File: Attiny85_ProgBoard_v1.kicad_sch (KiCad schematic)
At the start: 1 part, among them U1 ATtiny85V-10PU

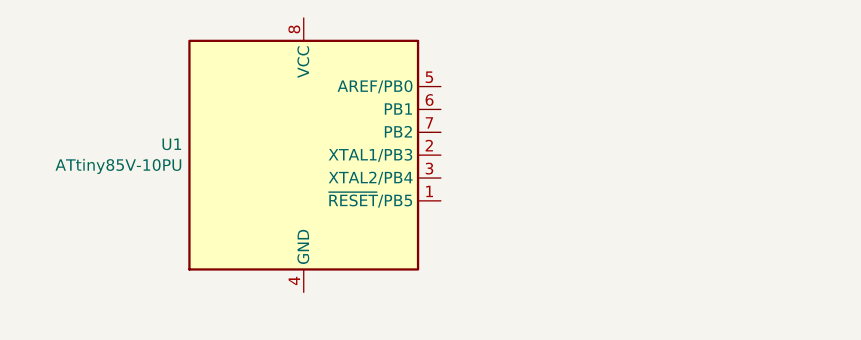
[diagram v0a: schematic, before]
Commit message: Designed PCB
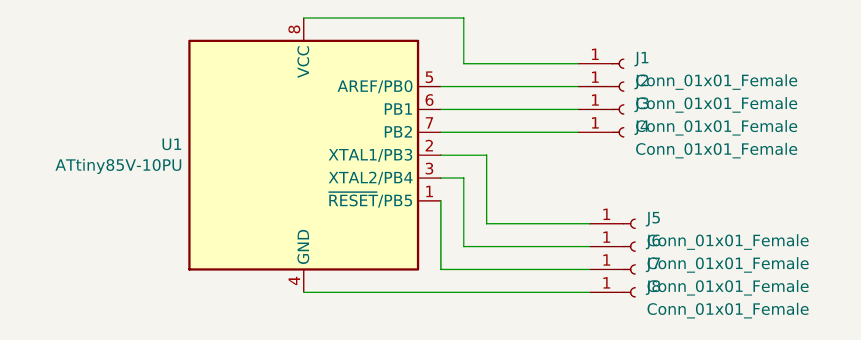
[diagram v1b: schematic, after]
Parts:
- added J1, J2, J3, J4, J5, J6, J7, J8: Conn_01x01_Female, Connector_Pin:PinHole_01x01, symbol Connector:Conn_01x01_Female
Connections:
- net at U1.1 (~{RESET}/PB5): now also J7.1 (Pin_1)
- net at U1.2 (XTAL1/PB3): now also J5.1 (Pin_1)
- net at U1.3 (XTAL2/PB4): now also J6.1 (Pin_1)
- net at U1.4 (GND): now also J8.1 (Pin_1)
- net at U1.5 (AREF/PB0): now also J2.1 (Pin_1)
- net at U1.6 (PB1): now also J3.1 (Pin_1)
- net at U1.7 (PB2): now also J4.1 (Pin_1)
- net at U1.8 (VCC): now also J1.1 (Pin_1)
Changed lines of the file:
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@@
 (kicad_sch (version 20230121) (generator eeschema)
   (paper "A4")
+  (wire (pts (xy 120.65 60.96) (xy 138.43 60.96))
+    (stroke (width 0) (type default))
+  )
+  (wire (pts (xy 135.89 71.12) (xy 151.13 71.12))
+    (stroke (width 0) (type default))
+  )
+  (wire (pts (xy 138.43 78.74) (xy 135.89 78.74))
+    (stroke (width 0) (type default))
+  )
+  (wire (pts (xy 135.89 88.9) (xy 152.4 88.9))
+    (stroke (width 0) (type default))
+  )
+  (wire (pts (xy 152.4 86.36) (xy 138.43 86.36))
+    (stroke (width 0) (type default))
+  )
+  (wire (pts (xy 135.89 76.2) (xy 140.97 76.2))
+    (stroke (width 0) (type default))
+  )
+  (wire (pts (xy 138.43 86.36) (xy 138.43 78.74))
+    (stroke (width 0) (type default))
+  )
+  (wire (pts (xy 135.89 73.66) (xy 151.13 73.66))
+    (stroke (width 0) (type default))
+  )
+  (wire (pts (xy 120.65 91.44) (xy 152.4 91.44))
+    (stroke (width 0) (type default))
+  )
+  (wire (pts (xy 140.97 83.82) (xy 152.4 83.82))
+    (stroke (width 0) (type default))
+  )
+  (wire (pts (xy 135.89 81.28) (xy 135.89 88.9))
+    (stroke (width 0) (type default))
+  )
+  (wire (pts (xy 138.43 66.04) (xy 138.43 60.96))
+    (stroke (width 0) (type default))
+  )
+  (wire (pts (xy 140.97 76.2) (xy 140.97 83.82))
+    (stroke (width 0) (type default))
+  )
+  (wire (pts (xy 151.13 66.04) (xy 138.43 66.04))
+    (stroke (width 0) (type default))
+  )
+  (wire (pts (xy 135.89 68.58) (xy 151.13 68.58))
+    (stroke (width 0) (type default))
+  )
   (symbol (lib_id "Attiny85_ProgBoard_v1-rescue:ATtiny85V-10PU-MCU_Microchip_ATtiny") (at 120.65 76.2 0) (unit 1)
     (in_bom yes) (on_board yes) (dnp no)
@@
         )
       )
+    )
+  )
+  (symbol (lib_id "Connector:Conn_01x01_Female") (at 157.48 88.9 0) (unit 1)
+    (in_bom yes) (on_board yes) (dnp no) (fields_autoplaced)
+    (property "Reference" "J7" (at 158.75 88.265 0)
+      (effects (font (size 1.27 1.27)) (justify left))
+    )
+    (property "Value" "Conn_01x01_Female" (at 158.75 90.805 0)
+      (effects (font (size 1.27 1.27)) (justify left))
+    )
+    (property "Footprint" "Connector_Pin:PinHole_01x01" (at 157.48 88.9 0)
+      (effects (font (size 1.27 1.27)) hide)
+    )
+    (property "Datasheet" "~" (at 157.48 88.9 0)
+      (effects (font (size 1.27 1.27)) hide)
+    )
+    (pin "1")
+    (instances
+      (project "Attiny85_ProgBoard_v1"
+        (path "/461172af-f3d0-444f-a1ea-3ea6bb3ec9d2"
+          (reference "J7") (unit 1)
+        )
+      )
+    )
+  )
+  (symbol (lib_id "Connector:Conn_01x01_Female") (at 156.21 73.66 0) (unit 1)
+    (in_bom yes) (on_board yes) (dnp no) (fields_autoplaced)
+    (property "Reference" "J4" (at 157.48 73.025 0)
+      (effects (font (size 1.27 1.27)) (justify left))
+    )
+    (property "Value" "Conn_01x01_Female" (at 157.48 75.565 0)
+      (effects (font (size 1.27 1.27)) (justify left))
+    )
+    (property "Footprint" "Connector_Pin:PinHole_01x01" (at 156.21 73.66 0)
+      (effects (font (size 1.27 1.27)) hide)
+    )
+    (property "Datasheet" "~" (at 156.21 73.66 0)
+      (effects (font (size 1.27 1.27)) hide)
+    )
+    (pin "1")
+    (instances
+      (project "Attiny85_ProgBoard_v1"
+        (path "/461172af-f3d0-444f-a1ea-3ea6bb3ec9d2"
+          (reference "J4") (unit 1)
+        )
+      )
+    )
+  )
+  (symbol (lib_id "Connector:Conn_01x01_Female") (at 156.21 66.04 0) (unit 1)
+    (in_bom yes) (on_board yes) (dnp no) (fields_autoplaced)
+    (property "Reference" "J1" (at 157.48 65.405 0)
+      (effects (font (size 1.27 1.27)) (justify left))
+    )
+    (property "Value" "Conn_01x01_Female" (at 157.48 67.945 0)
+      (effects (font (size 1.27 1.27)) (justify left))
+    )
+    (property "Footprint" "Connector_Pin:PinHole_01x01" (at 156.21 66.04 0)
+      (effects (font (size 1.27 1.27)) hide)
+    )
+    (property "Datasheet" "~" (at 156.21 66.04 0)
+      (effects (font (size 1.27 1.27)) hide)
+    )
+    (pin "1")
+    (instances
+      (project "Attiny85_ProgBoard_v1"
+        (path "/461172af-f3d0-444f-a1ea-3ea6bb3ec9d2"
+          (reference "J1") (unit 1)
+        )
+      )
+    )
+  )
+  (symbol (lib_id "Connector:Conn_01x01_Female") (at 157.48 83.82 0) (unit 1)
+    (in_bom yes) (on_board yes) (dnp no) (fields_autoplaced)
+    (property "Reference" "J5" (at 158.75 83.185 0)
+      (effects (font (size 1.27 1.27)) (justify left))
+    )
+    (property "Value" "Conn_01x01_Female" (at 158.75 85.725 0)
+      (effects (font (size 1.27 1.27)) (justify left))
+    )
+    (property "Footprint" "Connector_Pin:PinHole_01x01" (at 157.48 83.82 0)
+      (effects (font (size 1.27 1.27)) hide)
+    )
+    (property "Datasheet" "~" (at 157.48 83.82 0)
+      (effects (font (size 1.27 1.27)) hide)
+    )
+    (pin "1")
+    (instances
+      (project "Attiny85_ProgBoard_v1"
+        (path "/461172af-f3d0-444f-a1ea-3ea6bb3ec9d2"
+          (reference "J5") (unit 1)
+        )
+      )
+    )
+  )
+  (symbol (lib_id "Connector:Conn_01x01_Female") (at 157.48 86.36 0) (unit 1)
+    (in_bom yes) (on_board yes) (dnp no) (fields_autoplaced)
+    (property "Reference" "J6" (at 158.75 85.725 0)
+      (effects (font (size 1.27 1.27)) (justify left))
+    )
+    (property "Value" "Conn_01x01_Female" (at 158.75 88.265 0)
+      (effects (font (size 1.27 1.27)) (justify left))
+    )
+    (property "Footprint" "Connector_Pin:PinHole_01x01" (at 157.48 86.36 0)
+      (effects (font (size 1.27 1.27)) hide)
+    )
+    (property "Datasheet" "~" (at 157.48 86.36 0)
+      (effects (font (size 1.27 1.27)) hide)
+    )
+    (pin "1")
+    (instances
+      (project "Attiny85_ProgBoard_v1"
+        (path "/461172af-f3d0-444f-a1ea-3ea6bb3ec9d2"
+          (reference "J6") (unit 1)
+        )
+      )
+    )
+  )
+  (symbol (lib_id "Connector:Conn_01x01_Female") (at 157.48 91.44 0) (unit 1)
+    (in_bom yes) (on_board yes) (dnp no) (fields_autoplaced)
+    (property "Reference" "J8" (at 158.75 90.805 0)
+      (effects (font (size 1.27 1.27)) (justify left))
+    )
+    (property "Value" "Conn_01x01_Female" (at 158.75 93.345 0)
+      (effects (font (size 1.27 1.27)) (justify left))
+    )
+    (property "Footprint" "Connector_Pin:PinHole_01x01" (at 157.48 91.44 0)
+      (effects (font (size 1.27 1.27)) hide)
+    )
+    (property "Datasheet" "~" (at 157.48 91.44 0)
+      (effects (font (size 1.27 1.27)) hide)
+    )
+    (pin "1")
+    (instances
+      (project "Attiny85_ProgBoard_v1"
+        (path "/461172af-f3d0-444f-a1ea-3ea6bb3ec9d2"
+          (reference "J8") (unit 1)
+        )
+      )
+    )
+  )
+  (symbol (lib_id "Connector:Conn_01x01_Female") (at 156.21 68.58 0) (unit 1)
+    (in_bom yes) (on_board yes) (dnp no) (fields_autoplaced)
+    (property "Reference" "J2" (at 157.48 67.945 0)
+      (effects (font (size 1.27 1.27)) (justify left))
+    )
+    (property "Value" "Conn_01x01_Female" (at 157.48 70.485 0)
+      (effects (font (size 1.27 1.27)) (justify left))
+    )
+    (property "Footprint" "Connector_Pin:PinHole_01x01" (at 156.21 68.58 0)
+      (effects (font (size 1.27 1.27)) hide)
+    )
+    (property "Datasheet" "~" (at 156.21 68.58 0)
+      (effects (font (size 1.27 1.27)) hide)
+    )
+    (pin "1")
+    (instances
+      (project "Attiny85_ProgBoard_v1"
+        (path "/461172af-f3d0-444f-a1ea-3ea6bb3ec9d2"
+          (reference "J2") (unit 1)
+        )
+      )
+    )
+  )
+  (symbol (lib_id "Connector:Conn_01x01_Female") (at 156.21 71.12 0) (unit 1)
+    (in_bom yes) (on_board yes) (dnp no) (fields_autoplaced)
+    (property "Reference" "J3" (at 157.48 70.485 0)
+      (effects (font (size 1.27 1.27)) (justify left))
+    )
+    (property "Value" "Conn_01x01_Female" (at 157.48 73.025 0)
+      (effects (font (size 1.27 1.27)) (justify left))
+    )
+    (property "Footprint" "Connector_Pin:PinHole_01x01" (at 156.21 71.12 0)
+      (effects (font (size 1.27 1.27)) hide)
+    )
+    (property "Datasheet" "~" (at 156.21 71.12 0)
+      (effects (font (size 1.27 1.27)) hide)
+    )
+    (pin "1")
+    (instances
+      (project "Attiny85_ProgBoard_v1"
+        (path "/461172af-f3d0-444f-a1ea-3ea6bb3ec9d2"
+          (reference "J3") (unit 1)
+        )
+      )
